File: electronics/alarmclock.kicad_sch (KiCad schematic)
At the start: 41 parts, among them J1 Conn_01x02, J2 SWD, J3 SocketTop, J4 SocketBottem, J5 Conn_01x02, J6 Conn_01x05, J7 Conn_01x05, J8 RotaryEncoder, Q1 Backpower, SW2 Reset, U1 STM32L031F6P6, U2 74HCT595, U3 74HCT595, U4 AP2111H-3.3, Y2 32.768khz

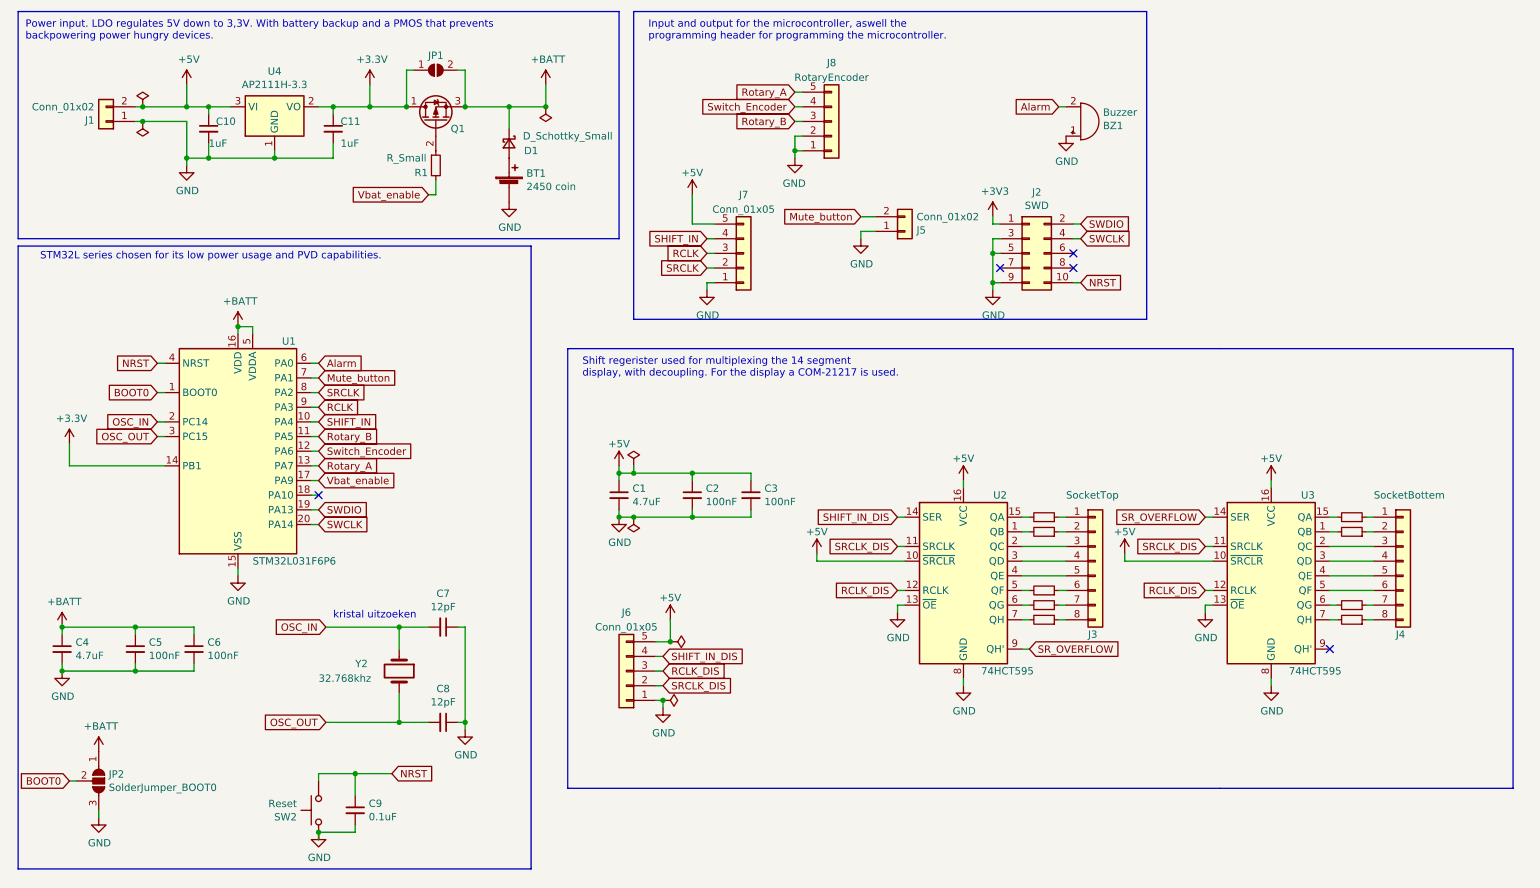
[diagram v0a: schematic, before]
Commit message: tape out
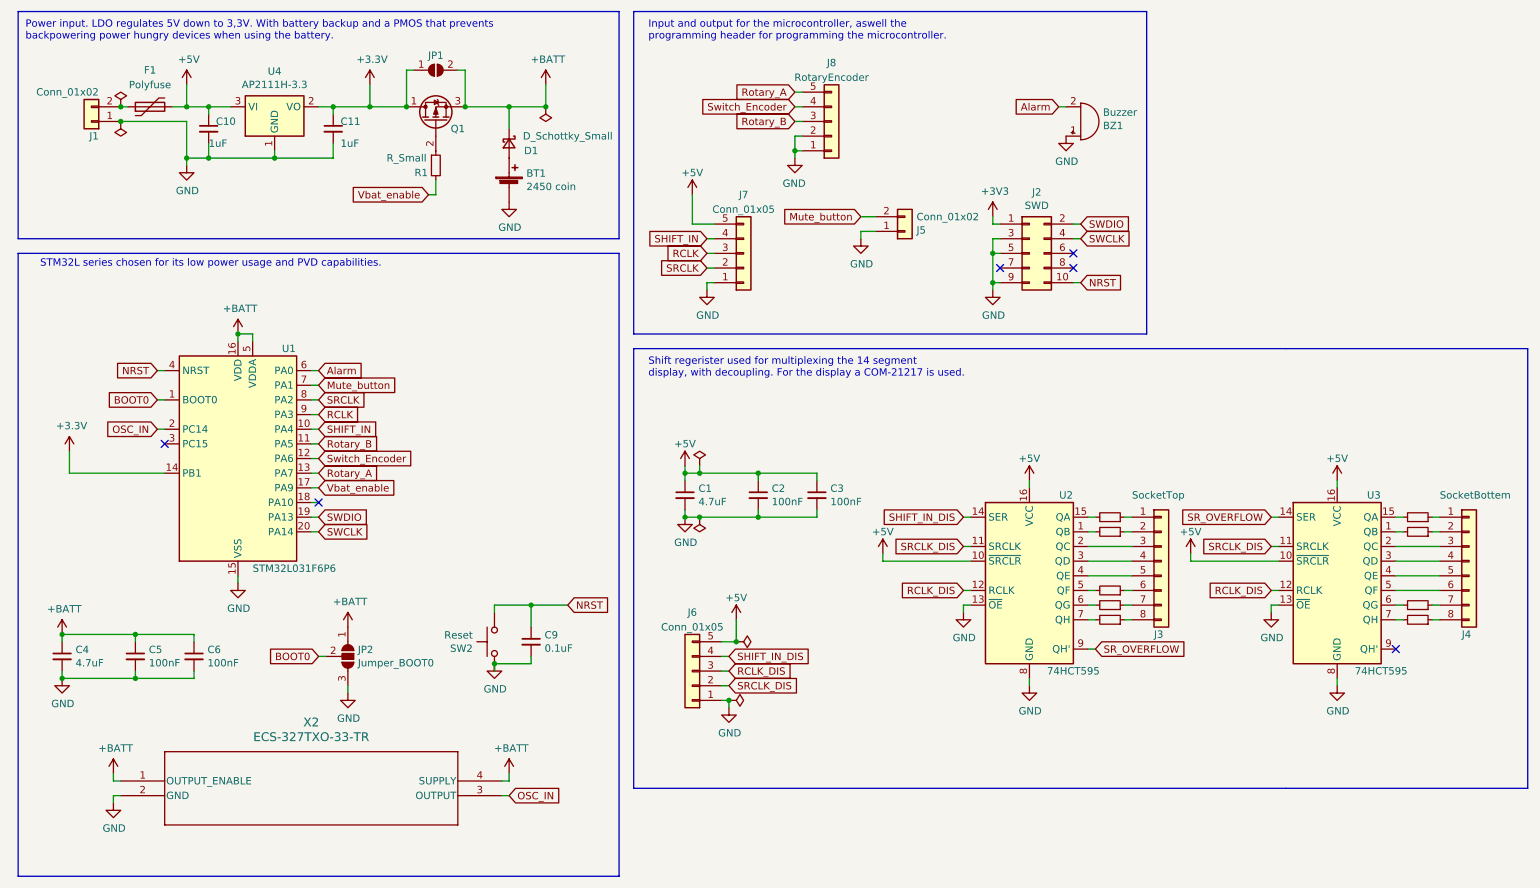
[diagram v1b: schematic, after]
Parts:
- removed C7, C8: 12pF, Capacitor_SMD:C_0805_2012Metric, symbol Device:C_Small
- removed Y2: 32.768khz, Crystal:Crystal_SMD_3215-2Pin_3.2x1.5mm, symbol Device:Crystal
- added F1: Polyfuse, Fuse:Fuse_1206_3216Metric, symbol Device:Polyfuse
- added X2: ECS-327TXO-33-TR, clockcyrstal:ECS-327_ECS, symbol clockcyrstal:ECS-327TXO-33-TR
- JP2: value SolderJumper_BOOT0 -> Jumper_BOOT0
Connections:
- net +5V: now also F1.2; no longer J1.2 (Pin_2)
- net +BATT: now also X2.1 (OUTPUT_ENABLE), X2.4 (SUPPLY)
- net GND: now also X2.2 (GND)
- net OSC_IN: now also X2.3 (OUTPUT)
- net OSC_OUT: no longer names the net of U1.3 (PC15)
- new net: F1.1, J1.2 (Pin_2)
- no-connect marks 5 -> 6
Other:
- note added: "Power input. LDO regulates 5V down to 3,3V. With battery backup and a PMOS that prevents backpowering power hungry devices when using the battery."
- note removed: "Power input. LDO regulates 5V down to 3,3V. With battery backup and a PMOS that prevents backpowering power hungry devices."
- note removed: "kristal uitzoeken"
- moved on the sheet: C1, C2, C3, C4, C5, C6, C9, J1, J3, J4, J6, JP2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
